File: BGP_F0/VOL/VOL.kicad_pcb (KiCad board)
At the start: 2 copper layers, 20 x 26 mm, 4 parts, among them J1 Conn_01x03_Female, J2 Conn_01x03_Female, P1 CONN_01X02

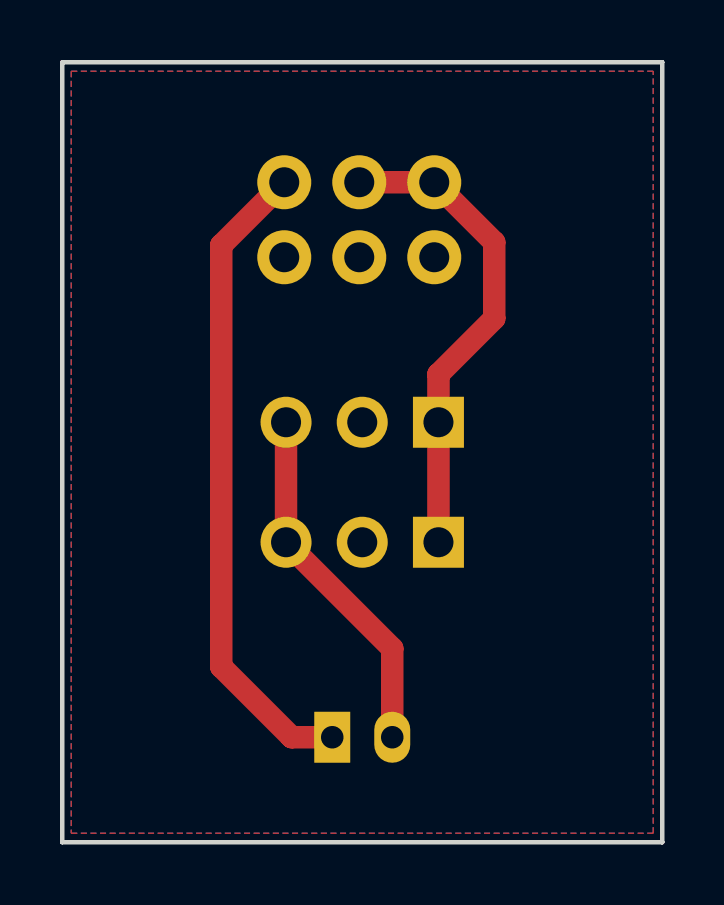
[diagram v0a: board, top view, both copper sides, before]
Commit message: Various
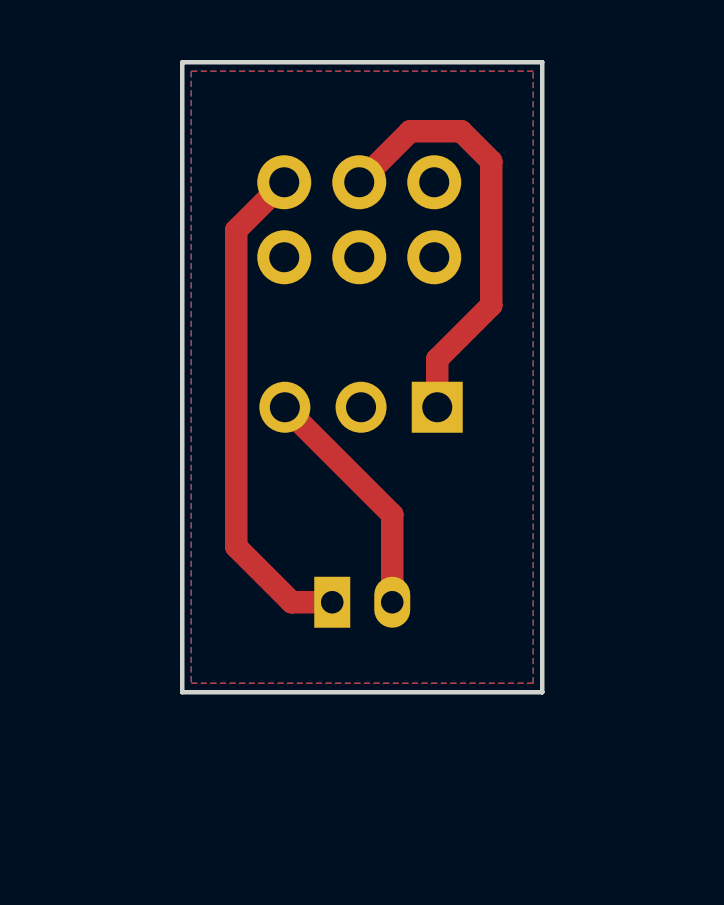
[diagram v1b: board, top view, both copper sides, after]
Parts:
- removed J2: Conn_01x03_Female, Pin_Headers:Pin_Header_Straight_1x03_Pitch2.54mm
- moved P1 4.50 mm to (147.0, 94.0)
- moved J1 0.50 mm to (150.5, 87.5)
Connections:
- J1 pad 1: Net-(J1-Pad1) -> Net-(C1-Pad1)
- RV1 pad 2: Net-(J1-Pad1) -> Net-(C1-Pad1)
- RV1 pad 3: Net-(J1-Pad1) -> Net-(RV1-Pad3)
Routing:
- net Net-(J1-Pad1): track 16.1 -> 0.00 mm
- net Net-(C1-Pad1): track 0.00 -> 14.5 mm
- net /VOL_1: track 21.7 -> 16.8 mm
- net /VOL_3: track 12.0 -> 7.98 mm
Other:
- board size 20 x 26 mm -> 12 x 21 mm
